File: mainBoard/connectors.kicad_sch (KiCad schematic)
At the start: 37 parts, among them J10 Conn_01x06, J11 Conn_01x07, J12 Conn_01x04, J13 Conn_01x04, J15 Conn_02x05_Odd_Even, J16 Conn_01x02, J17 Conn_01x06, J7 Conn_01x02, J8 Conn_01x02, J9 Conn_01x02, K1 Relay_SPDT, Q3 IRLML6244TRPBF, Q4 IRLML6244TRPBF, Q5 IRLML6244TRPBF, Q6 IRLML6244TRPBF, Q7 IRLML6244TRPBF

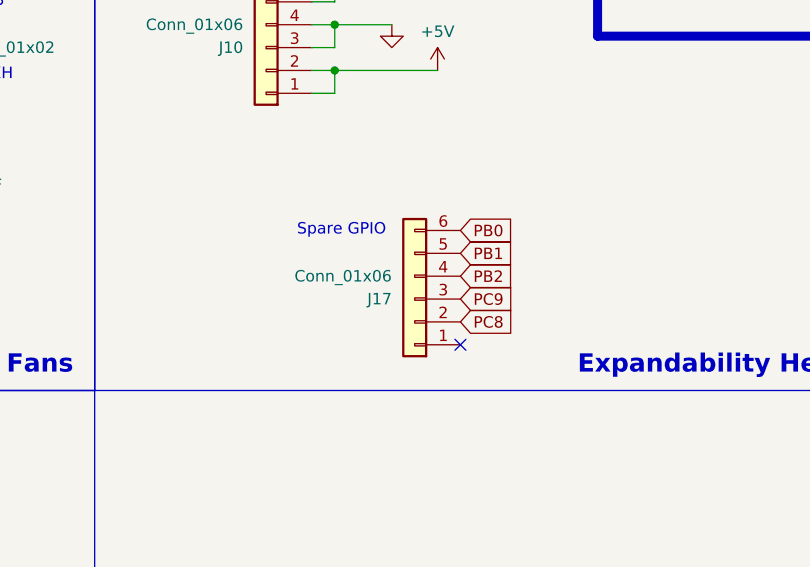
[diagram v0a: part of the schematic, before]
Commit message: board routing nearly complete
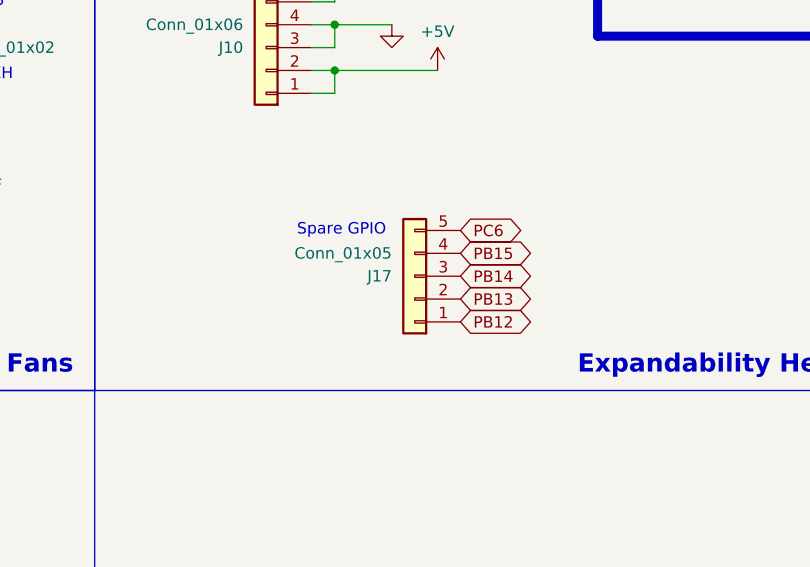
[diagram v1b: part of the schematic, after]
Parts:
- J17: value Conn_01x06 -> Conn_01x05; footprint Connector_PinHeader_2.54mm:PinHeader_1x06_P2.54mm_Vertical -> Connector_PinHeader_2.54mm:PinHeader_1x05_P2.54mm_Vertical; symbol Connector_Generic:Conn_01x06 -> Connector_Generic:Conn_01x05
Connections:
- net PB12: now reaches J17.1 (Pin_1)
- removed net PB0: J17.6 (Pin_6)
- net PB1 renamed PC6
- net PB2 renamed PB15
- net PC8 renamed PB13
- net PC9 renamed PB14
- no-connect marks 3 -> 2
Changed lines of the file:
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@@
 	)
 	(no_connect
-		(at 152.4 207.01)
-	)
-	(no_connect
 		(at 274.32 104.14)
 	)
@@
 		)
 	)
-	(global_label "PB1"
+	(global_label "Fan2"
 		(shape input)
-		(at 152.4 196.85 0)
+		(at 52.07 137.16 180)
 		(fields_autoplaced yes)
 		(effects
@@
 				(size 1.27 1.27)
 			)
-			(justify left)
+			(justify right)
 		)
 		(property "Intersheetrefs" "${INTERSHEET_REFS}"
-			(at 159.1347 196.85 0)
+			(at 44.4887 137.16 0)
 			(hide yes)
 			(show_name no)
@@
 					(size 1.27 1.27)
 				)
-				(justify left)
+				(justify right)
 			)
 		)
 	)
-	(global_label "Fan2"
+	(global_label "KP_Row2"
 		(shape input)
-		(at 52.07 137.16 180)
+		(at 138.43 67.31 0)
 		(fields_autoplaced yes)
 		(effects
@@
 				(size 1.27 1.27)
 			)
-			(justify right)
+			(justify left)
 		)
 		(property "Intersheetrefs" "${INTERSHEET_REFS}"
-			(at 44.4887 137.16 0)
+			(at 149.8818 67.31 0)
 			(hide yes)
 			(show_name no)
@@
 					(size 1.27 1.27)
 				)
-				(justify right)
+				(justify left)
 			)
 		)
 	)
-	(global_label "KP_Row2"
-		(shape input)
-		(at 138.43 67.31 0)
+	(global_label "PB12"
+		(shape bidirectional)
+		(at 152.4 204.47 0)
 		(fields_autoplaced yes)
 		(effects
@@
 		)
 		(property "Intersheetrefs" "${INTERSHEET_REFS}"
-			(at 149.8818 67.31 0)
+			(at 161.4555 204.47 0)
 			(hide yes)
 			(show_name no)
@@
 		)
 	)
-	(global_label "PB0"
-		(shape input)
-		(at 152.4 194.31 0)
+	(global_label "PB13"
+		(shape bidirectional)
+		(at 152.4 201.93 0)
 		(fields_autoplaced yes)
 		(effects
@@
 		)
 		(property "Intersheetrefs" "${INTERSHEET_REFS}"
-			(at 159.1347 194.31 0)
+			(at 161.4555 201.93 0)
 			(hide yes)
 			(show_name no)
@@
 		)
 	)
+	(global_label "PC6"
+		(shape bidirectional)
+		(at 152.4 194.31 0)
+		(fields_autoplaced yes)
+		(effects
+			(font
+				(size 1.27 1.27)
+			)
+			(justify left)
+		)
+		(property "Intersheetrefs" "${INTERSHEET_REFS}"
+			(at 160.246 194.31 0)
+			(hide yes)
+			(show_name no)
+			(do_not_autoplace no)
+			(effects
+				(font
+					(size 1.27 1.27)
+				)
+				(justify left)
+			)
+		)
+	)
 	(global_label "Conv_Fan"
 		(shape input)
@@
 		)
 	)
-	(global_label "KP_Row3"
-		(shape input)
-		(at 138.43 64.77 0)
-		(fields_autoplaced yes)
-		(effects
-			(font
-				(size 1.27 1.27)
-			)
-			(justify left)
-		)
-		(property "Intersheetrefs" "${INTERSHEET_REFS}"
-			(at 149.8818 64.77 0)
-			(hide yes)
-			(show_name no)
-			(do_not_autoplace no)
-			(effects
-				(font
-					(size 1.27 1.27)
-				)
-				(justify left)
-			)
-		)
-	)
-	(global_label "PB2"
-		(shape input)
-		(at 152.4 199.39 0)
+	(global_label "PB15"
+		(shape bidirectional)
+		(at 152.4 196.85 0)
 		(fields_autoplaced yes)
 		(effects
@@
 		)
 		(property "Intersheetrefs" "${INTERSHEET_REFS}"
-			(at 159.1347 199.39 0)
+			(at 161.4555 196.85 0)
 			(hide yes)
 			(show_name no)
@@
 		)
 	)
-	(global_label "PC8"
+	(global_label "KP_Row3"
 		(shape input)
-		(at 152.4 204.47 0)
+		(at 138.43 64.77 0)
 		(fields_autoplaced yes)
 		(effects
@@
 		)
 		(property "Intersheetrefs" "${INTERSHEET_REFS}"
-			(at 159.1347 204.47 0)
+			(at 149.8818 64.77 0)
 			(hide yes)
 			(show_name no)
@@
 		)
 	)
-	(global_label "PC9"
-		(shape input)
-		(at 152.4 201.93 0)
+	(global_label "PB14"
+		(shape bidirectional)
+		(at 152.4 199.39 0)
 		(fields_autoplaced yes)
 		(effects
@@
 		)
 		(property "Intersheetrefs" "${INTERSHEET_REFS}"
-			(at 159.1347 201.93 0)
+			(at 161.4555 199.39 0)
 			(hide yes)
 			(show_name no)
@@
 	)
 	(symbol
-		(lib_id "Connector_Generic:Conn_01x06")
-		(at 147.32 201.93 180)
+		(lib_id "Connector_Generic:Conn_01x05")
+		(at 147.32 199.39 180)
 		(unit 1)
 		(body_style 1)
@@
 		(dnp no)
 		(property "Reference" "J17"
-			(at 144.78 201.9301 0)
+			(at 144.78 199.3901 0)
 			(show_name no)
 			(do_not_autoplace no)
@@
 			)
 		)
-		(property "Value" "Conn_01x06"
-			(at 144.78 199.3901 0)
+		(property "Value" "Conn_01x05"
+			(at 144.78 196.8501 0)
 			(show_name no)
 			(do_not_autoplace no)
@@
 			)
 		)
-		(property "Footprint" "Connector_PinHeader_2.54mm:PinHeader_1x06_P2.54mm_Vertical"
-			(at 147.32 201.93 0)
+		(property "Footprint" "Connector_PinHeader_2.54mm:PinHeader_1x05_P2.54mm_Vertical"
+			(at 147.32 199.39 0)
 			(hide yes)
 			(show_name no)
@@
 		)
 		(property "Datasheet" ""
-			(at 147.32 201.93 0)
+			(at 147.32 199.39 0)
 			(hide yes)
 			(show_name no)
@@
 			)
 		)
-		(property "Description" "Generic connector, single row, 01x06, script generated (kicad-library-utils/schlib/autogen/connector/)"
-			(at 147.32 201.93 0)
+		(property "Description" "Generic connector, single row, 01x05, script generated (kicad-library-utils/schlib/autogen/connector/)"
+			(at 147.32 199.39 0)
 			(hide yes)
 			(show_name no)
@@
 		(pin "2"
 		)
-		(pin "6"
-		)
 		(pin "5"
